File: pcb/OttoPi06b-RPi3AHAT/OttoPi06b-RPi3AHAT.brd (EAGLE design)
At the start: 56 x 65 mm, 31 parts

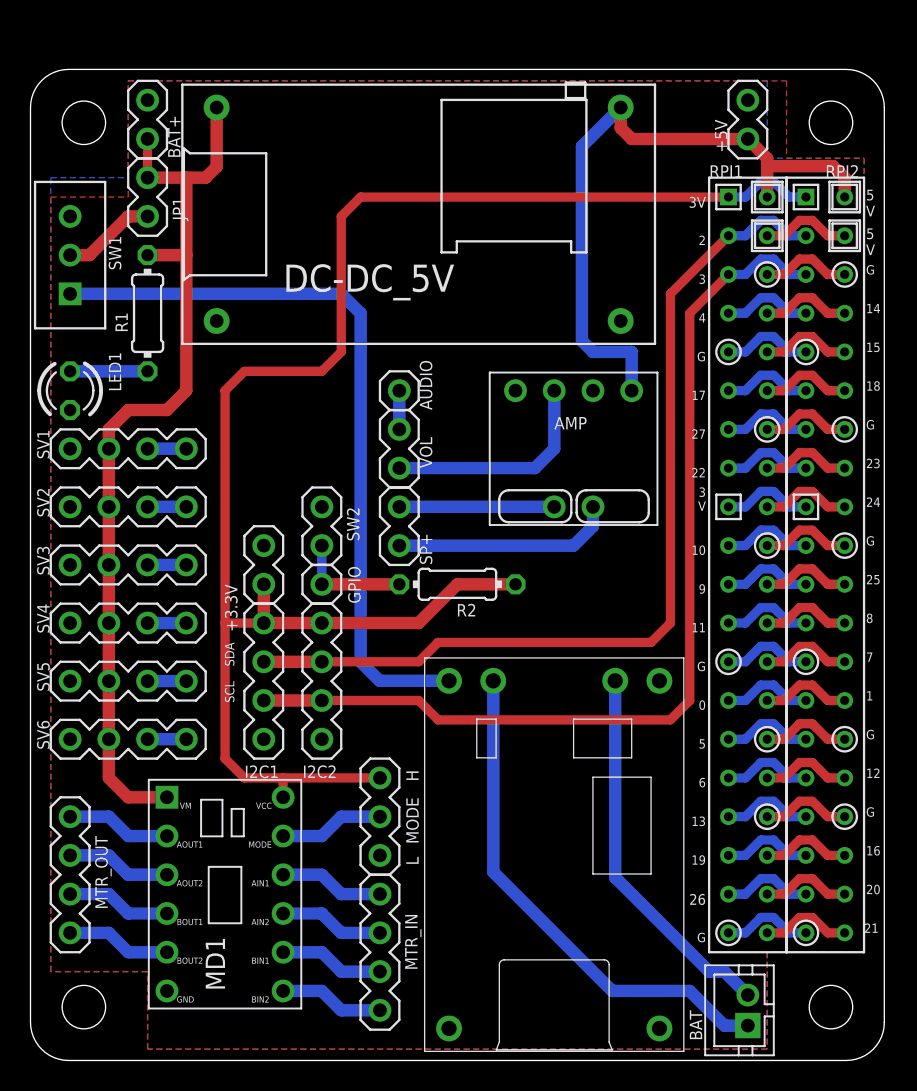
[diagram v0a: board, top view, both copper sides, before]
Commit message: update
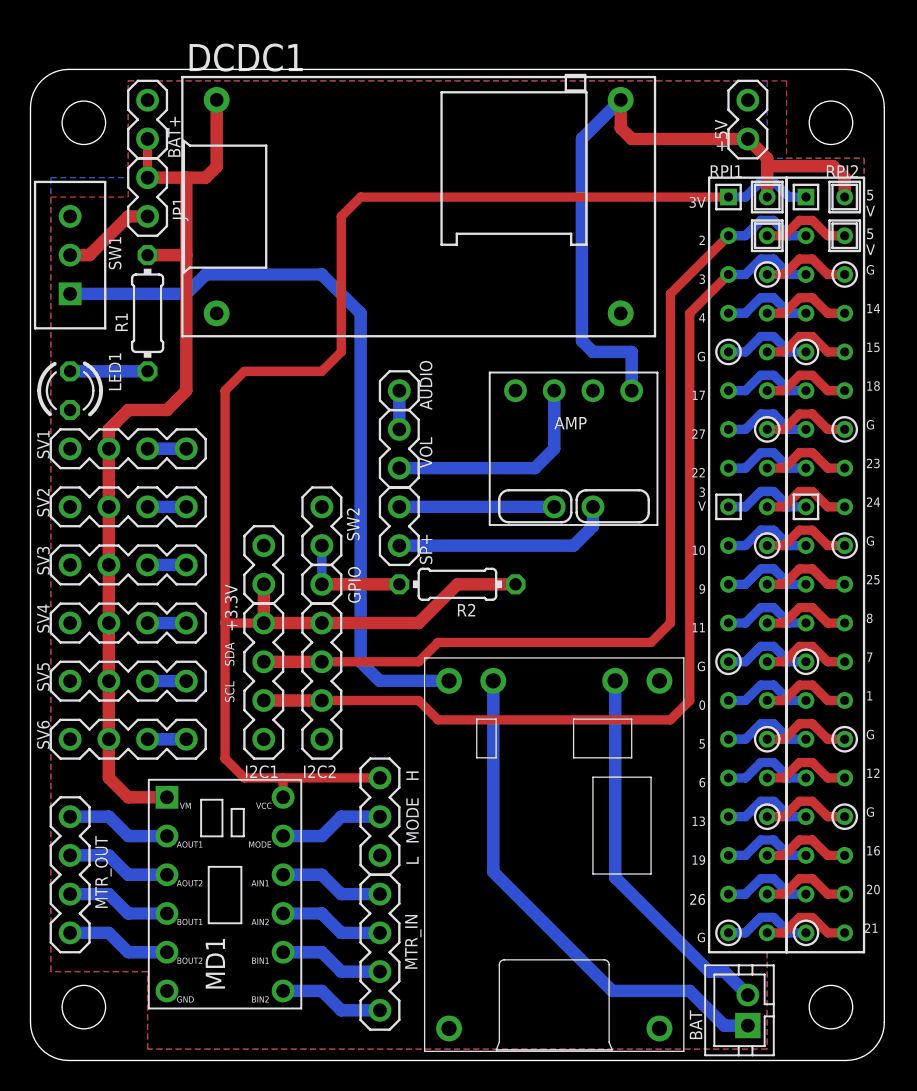
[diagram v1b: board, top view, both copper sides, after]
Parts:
- removed DC-DC_5V: (no value), ytani1:DCDC-5V_28V-2A
- added DCDC1: +5V, ytani1:DCDC-MT3608-MOD2-USB
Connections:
- net +5V: now also DCDC1.VOUT+; no longer DC-DC_5V.VOUT+
- net BAT+: now also DCDC1.VIN+; no longer DC-DC_5V.VIN+
- net GND: now also DCDC1.VIN-, DCDC1.VOUT-; no longer DC-DC_5V.VIN-, DC-DC_5V.VOUT-
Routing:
- net BAT+1: track 48.8 -> 49.8 mm
- net +5V: track 43.4 -> 44.4 mm
- net BAT+: track 61.1 -> 61.6 mm
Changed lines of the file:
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@@
 </autorouter>
 <elements>
-<element name="DC-DC_5V" library="ytani1" package="DCDC-5V_28V-2A" value="" x="-2.54" y="23" smashed="yes">
-<attribute name="NAME" x="-11.43" y="17.92" size="1.778" layer="25"/>
-<attribute name="URL_AMAZON" value="https://www.amazon.co.jp/gp/product/B01D0WSBGY/" x="-2.54" y="23" size="1.778" layer="27" display="off"/>
-<attribute name="VALUE" x="2.54" y="31.89" size="1.778" layer="27"/>
-</element>
 <element name="BAT" library="ytani1" package="JST-PH2" value="" x="19.05" y="-29.21" smashed="yes" rot="R90">
 <attribute name="NAME" x="15.24" y="-29.21" size="0.8128" layer="25" rot="R270"/>
@@
 <attribute name="VALUE" x="-10.16" y="-4.191" size="1.27" layer="27" ratio="10"/>
 </element>
+<element name="DCDC1" library="ytani1" package="DCDC-MT3608-MOD2-USB" value="+5V" x="-2.54" y="23.5" smashed="yes">
+<attribute name="AMAZON_URL" value="https://www.amazon.co.jp/gp/product/B01D0WSBGY/" x="-2.54" y="23.5" size="1.778" layer="27" display="off"/>
+<attribute name="NAME" x="-17.78" y="32.39" size="1.778" layer="25"/>
+<attribute name="VALUE" x="2.54" y="32.39" size="1.778" layer="27"/>
+</element>
 </elements>
 <signals>
@@
 <contactref element="CHG1" pad="OUT-"/>
 <contactref element="LED1" pad="K"/>
-<contactref element="DC-DC_5V" pad="VIN-"/>
-<contactref element="DC-DC_5V" pad="VOUT-"/>
-<contactref element="+5V" pad="2"/>
 <polygon width="0.15" layer="16">
 <vertex x="-26.67" y="25.4"/>
@@
 <contactref element="SW2" pad="1"/>
 <contactref element="SW1" pad="3"/>
+<contactref element="DCDC1" pad="VIN-"/>
+<contactref element="+5V" pad="2"/>
+<contactref element="DCDC1" pad="VOUT-"/>
 </signal>
 <signal name="BAT+">
-<contactref element="DC-DC_5V" pad="VIN+"/>
 <contactref element="R1" pad="2"/>
 <contactref element="BAT+" pad="1"/>
@@
 <wire x1="-17.78" y1="20.32" x2="-17.78" y2="11.43" width="0.8128" layer="1"/>
 <wire x1="-22.86" y1="8.89" x2="-22.86" y2="7.62" width="0.8128" layer="1"/>
-<wire x1="-15.79" y1="26.12" x2="-15.79" y2="30" width="0.8128" layer="1"/>
 <wire x1="-20.32" y1="25.4" x2="-20.32" y2="27.94" width="0.6096" layer="1"/>
-<wire x1="-15.79" y1="26.12" x2="-16.51" y2="25.4" width="0.8128" layer="1"/>
+<wire x1="-16.51" y1="25.4" x2="-15.79" y2="26.12" width="0.8128" layer="1"/>
 <wire x1="-16.51" y1="25.4" x2="-17.78" y2="25.4" width="0.8128" layer="1"/>
+<contactref element="DCDC1" pad="VIN+"/>
+<wire x1="-15.79" y1="26.12" x2="-15.79" y2="30.5" width="0.8128" layer="1"/>
 </signal>
 <signal name="+5V">
-<contactref element="DC-DC_5V" pad="VOUT+"/>
 <contactref element="+5V" pad="1"/>
 <contactref element="RPI2" pad="2"/>
@@
 <wire x1="24.6474" y1="26.1526" x2="20.32" y2="26.1526" width="0.8128" layer="1"/>
 <wire x1="20.32" y1="24.13" x2="20.32" y2="26.1526" width="0.8128" layer="1"/>
-<wire x1="10.71" y1="30" x2="10.71" y2="28.66" width="0.8128" layer="1"/>
-<wire x1="10.71" y1="28.66" x2="11.43" y2="27.94" width="0.8128" layer="1"/>
-<wire x1="11.43" y1="27.94" x2="19.05" y2="27.94" width="0.8128" layer="1"/>
+<wire x1="19.05" y1="27.94" x2="11.43" y2="27.94" width="0.8128" layer="1"/>
 <contactref element="AMP" pad="V+"/>
-<wire x1="8.17" y1="27.46" x2="10.71" y2="30" width="0.8128" layer="16"/>
 <wire x1="11.43" y1="11.43" x2="11.43" y2="13.97" width="0.8128" layer="16"/>
 <wire x1="11.43" y1="13.97" x2="8.89" y2="13.97" width="0.8128" layer="16"/>
 <wire x1="8.89" y1="13.97" x2="8.17" y2="14.69" width="0.8128" layer="16"/>
-<wire x1="8.17" y1="14.69" x2="8.17" y2="27.46" width="0.8128" layer="16"/>
+<contactref element="DCDC1" pad="VOUT+"/>
+<wire x1="11.43" y1="27.94" x2="10.71" y2="28.66" width="0.8128" layer="1"/>
+<wire x1="10.71" y1="28.66" x2="10.71" y2="30.5" width="0.8128" layer="1"/>
+<wire x1="8.17" y1="27.96" x2="10.71" y2="30.5" width="0.8128" layer="16"/>
+<wire x1="8.17" y1="14.69" x2="8.17" y2="27.96" width="0.8128" layer="16"/>
 </signal>
 <signal name="BAT+1">
 <contactref element="CHG1" pad="OUT+"/>
 <contactref element="SW1" pad="1"/>
-<wire x1="-25.4" y1="17.78" x2="-7.62" y2="17.78" width="0.8128" layer="16"/>
-<wire x1="-6.35" y1="16.51" x2="-7.62" y2="17.78" width="0.8128" layer="16"/>
 <wire x1="-0.55" y1="-7.6" x2="-5.1" y2="-7.6" width="0.8128" layer="16"/>
 <wire x1="-5.1" y1="-7.6" x2="-6.35" y2="-6.35" width="0.8128" layer="16"/>
-<wire x1="-6.35" y1="-6.35" x2="-6.35" y2="16.51" width="0.8128" layer="16"/>
+<wire x1="-6.35" y1="16.51" x2="-6.35" y2="-6.35" width="0.8128" layer="16"/>
+<wire x1="-25.4" y1="17.78" x2="-17.78" y2="17.78" width="0.8128" layer="16"/>
+<wire x1="-17.78" y1="17.78" x2="-16.51" y2="19.05" width="0.8128" layer="16"/>
+<wire x1="-16.51" y1="19.05" x2="-8.89" y2="19.05" width="0.8128" layer="16"/>
+<wire x1="-8.89" y1="19.05" x2="-6.35" y2="16.51" width="0.8128" layer="16"/>
 </signal>
 <signal name="N$3">
